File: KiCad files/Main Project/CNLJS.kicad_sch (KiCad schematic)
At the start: 0 parts

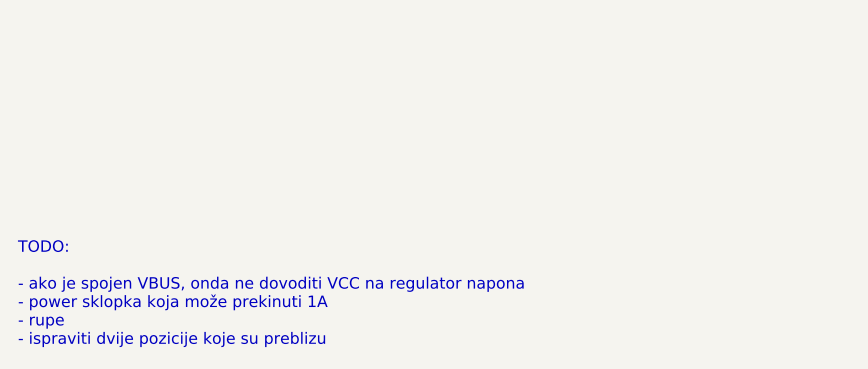
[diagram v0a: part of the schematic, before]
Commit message: update
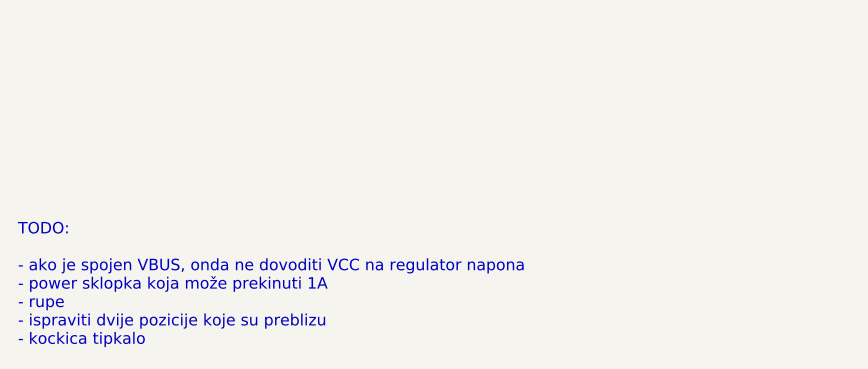
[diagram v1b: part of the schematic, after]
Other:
- note added: "TODO: - ako je spojen VBUS, onda ne dovoditi VCC na regulator napona - power sklopka koja može prekinuti 1A - rupe - ispraviti dvije pozicije koje su preblizu - kockica tipkalo"
- note removed: "TODO: - ako je spojen VBUS, onda ne dovoditi VCC na regulator napona - power sklopka koja može prekinuti 1A - rupe - ispraviti dvije pozicije koje su preblizu"
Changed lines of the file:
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@@
     (effects (font (size 1.27 1.27)) (justify left bottom))
   )
-  (text "TODO:\n\n- ako je spojen VBUS, onda ne dovoditi VCC na regulator napona\n- power sklopka koja može prekinuti 1A\n- rupe\n- ispraviti dvije pozicije koje su preblizu"
+  (text "TODO:\n\n- ako je spojen VBUS, onda ne dovoditi VCC na regulator napona\n- power sklopka koja može prekinuti 1A\n- rupe\n- ispraviti dvije pozicije koje su preblizu\n- kockica tipkalo"
     (at 18.415 186.055 0)
     (effects (font (size 1.27 1.27)) (justify left bottom))

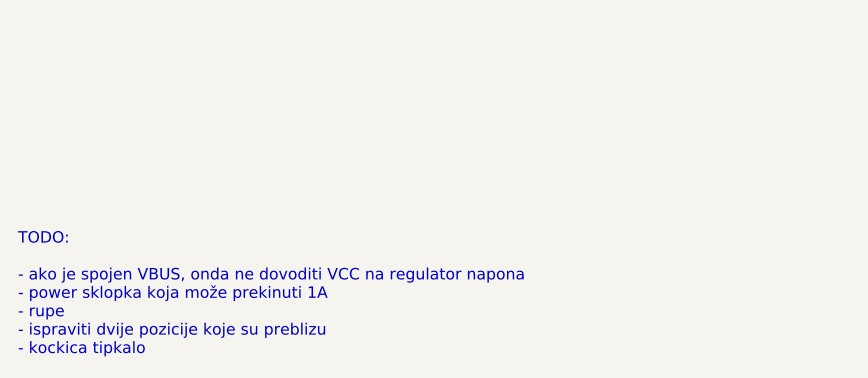
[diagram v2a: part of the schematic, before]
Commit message: update
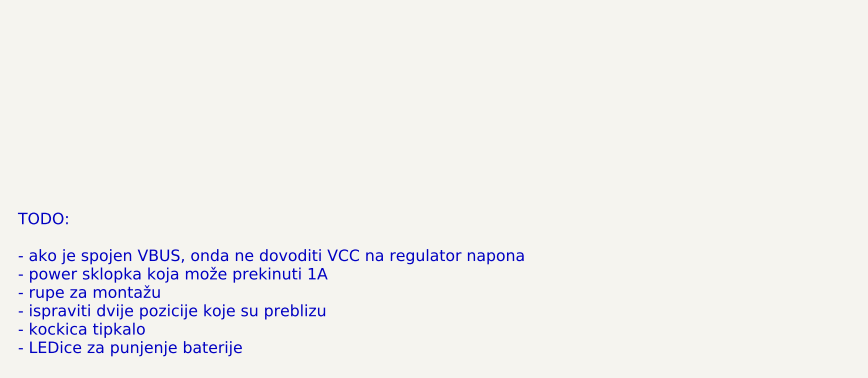
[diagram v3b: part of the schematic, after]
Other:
- note added: "TODO: - ako je spojen VBUS, onda ne dovoditi VCC na regulator napona - power sklopka koja može prekinuti 1A - rupe za montažu - ispraviti dvije pozicije koje su preblizu - kockica tipkalo - LEDice za punjenje baterije"
- note removed: "TODO: - ako je spojen VBUS, onda ne dovoditi VCC na regulator napona - power sklopka koja može prekinuti 1A - rupe - ispraviti dvije pozicije koje su preblizu - kockica tipkalo"
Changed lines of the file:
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@@
     (effects (font (size 1.27 1.27)) (justify left bottom))
   )
-  (text "TODO:\n\n- ako je spojen VBUS, onda ne dovoditi VCC na regulator napona\n- power sklopka koja može prekinuti 1A\n- rupe\n- ispraviti dvije pozicije koje su preblizu\n- kockica tipkalo"
+  (text "TODO:\n\n- ako je spojen VBUS, onda ne dovoditi VCC na regulator napona\n- power sklopka koja može prekinuti 1A\n- rupe za montažu\n- ispraviti dvije pozicije koje su preblizu\n- kockica tipkalo\n- LEDice za punjenje baterije"
     (at 18.415 186.055 0)
     (effects (font (size 1.27 1.27)) (justify left bottom))
